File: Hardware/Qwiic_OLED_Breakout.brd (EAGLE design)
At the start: 20.3 x 29.2 mm, 26 parts

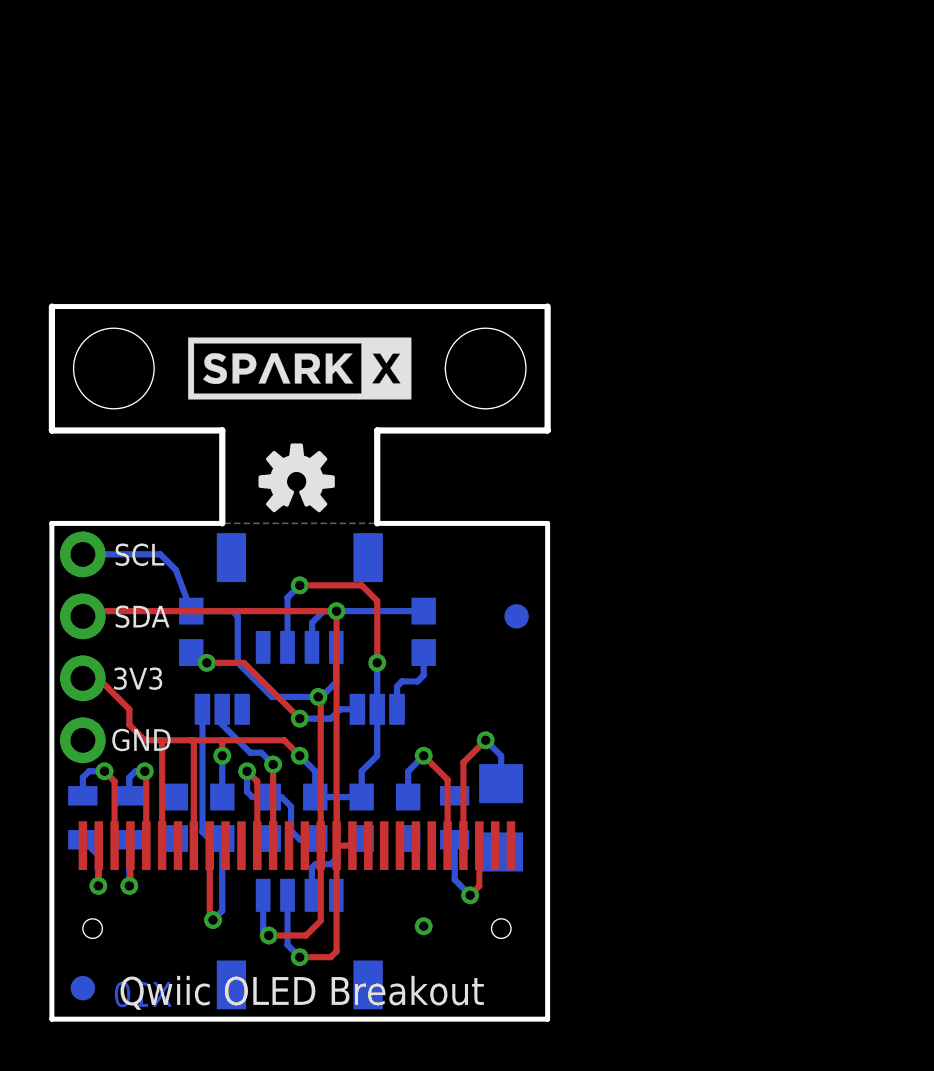
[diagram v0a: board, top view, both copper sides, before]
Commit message: Mold V2
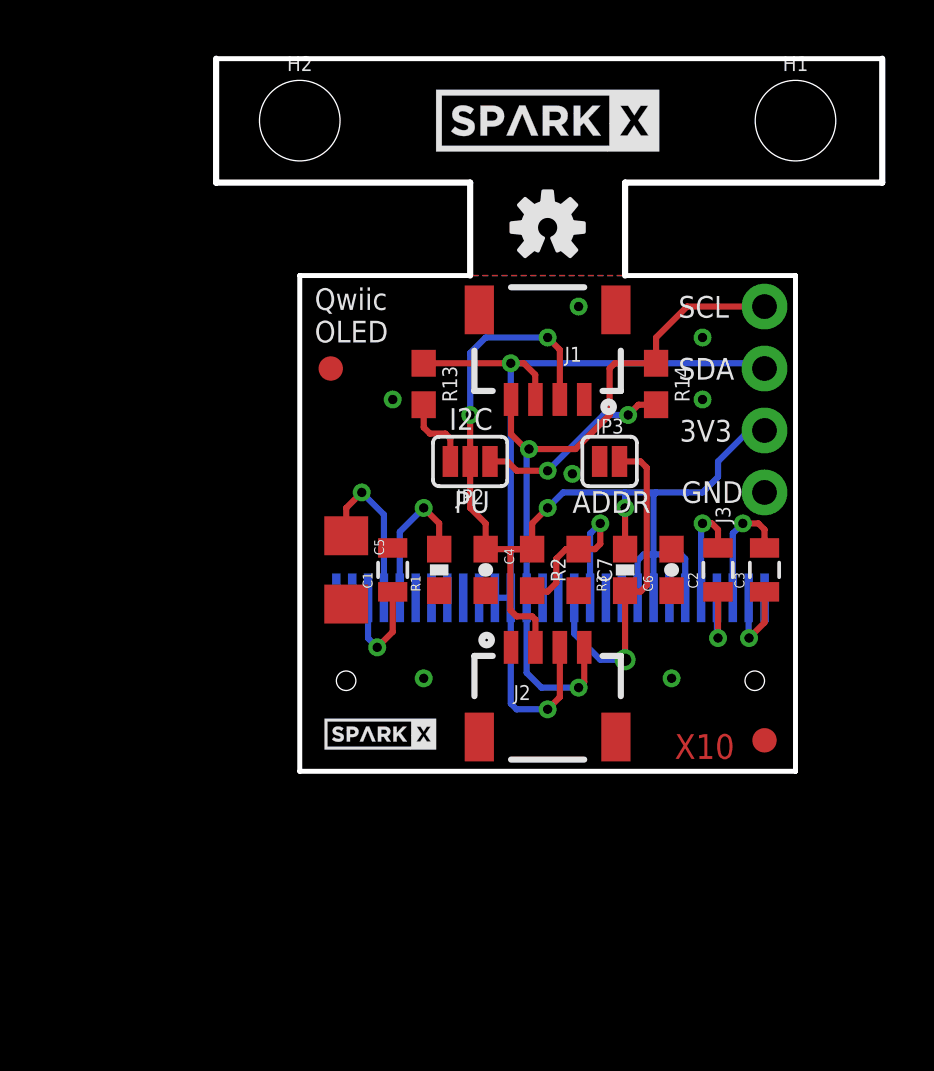
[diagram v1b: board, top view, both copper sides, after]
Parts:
- removed JP1: JUMPER-SMT_3_1-NC_PASTE_SILK, SparkFun-Jumpers:SMT-JUMPER_3_1-NC_PASTE_SILK
- added JP3: (no value), SparkFun-Jumpers:SMT-JUMPER_2_NO_SILK
- added U$3: SPARKX-LOGO2, SparkX:SPARKX-TINY
- moved FRAME1 35.6 mm to (17.8, -19.1), flipped to the bottom
- moved C3 29.7 mm to (19.1, 8.26), flipped to the top
- moved FID1 29.7 mm to (19.1, 1.27), flipped to the top
- moved H1 29.7 mm to (20.3, 26.7), flipped to the top
- moved J3 29.7 mm to (19.1, 11.4), flipped to the top
- moved OLED1 29.7 mm to (19.1, 7.11), flipped to the bottom
- moved C2 26.2 mm to (17.1, 8.26), flipped to the top
- moved C6 22.7 mm to (15.2, 8.26), flipped to the top
- moved R14 21.6 mm to (14.6, 15.9), flipped to the top
- moved R3 19.4 mm to (13.3, 8.26), flipped to the top
- moved C7 16.3 mm to (11.4, 8.26), flipped to the top
- moved LOGO3 14.6 mm to (10.2, 22.3)
- moved J1 14.4 mm to (10.2, 15.2), flipped to the top
- moved J2 14.4 mm to (10.2, 5.08), flipped to the top
- moved U$1 14.4 mm to (10.2, 26.7), flipped to the top
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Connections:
- removed net VDD_PU1: JP1.3, OLED1.9, R3.1
- net D/C: now also JP3.2, R3.1; no longer JP1.2
- net GND: now also JP3.1; no longer JP1.1
- net VDD: now also OLED1.9
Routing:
- net VDD_PU1: track 12.6 -> 0.00 mm, vias 1 -> 0
- net D/C: track 6.72 -> 13.9 mm
- net VDD: track 45.7 -> 46.7 mm
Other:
- board size 20.3 x 29.2 mm -> 27.3 x 29.2 mm
